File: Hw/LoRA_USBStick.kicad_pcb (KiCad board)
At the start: 2 copper layers, 61.5 x 18.7 mm, 17 parts, among them J10 USB_B, J4 SWD, SW1 RST, U1 ATSAMD21E, U2 RFM95W-868S2, U7 AP2114H-3.3TRG1

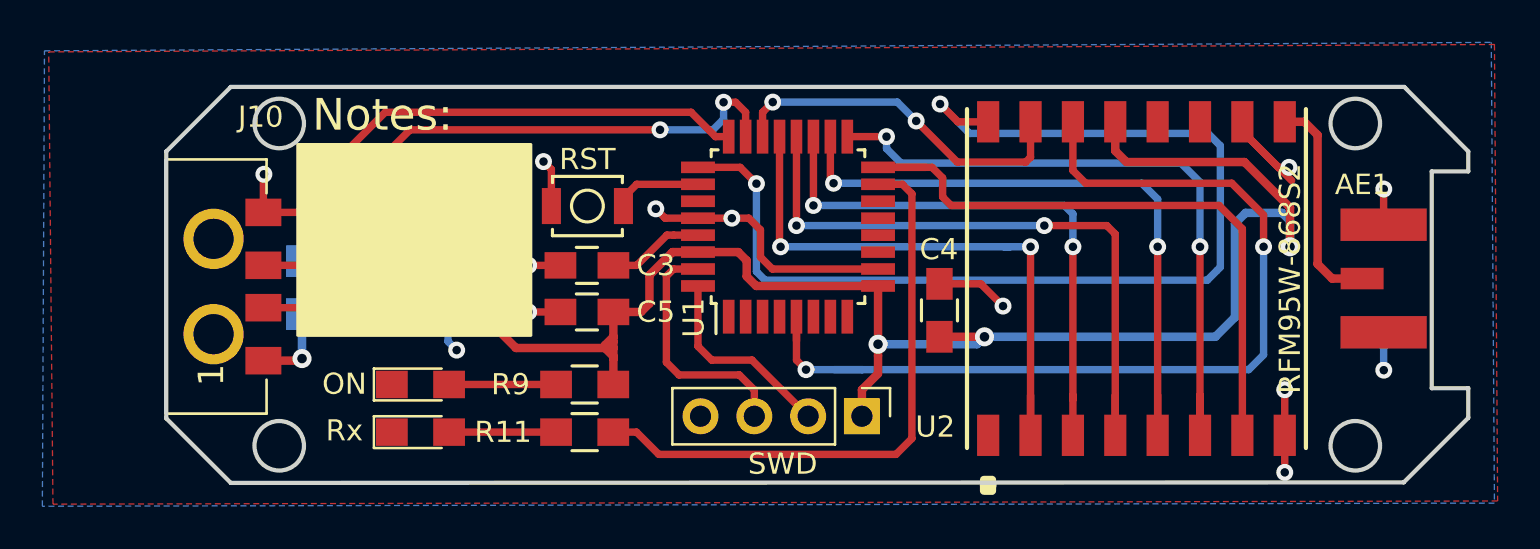
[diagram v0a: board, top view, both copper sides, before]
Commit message: Add v2.0
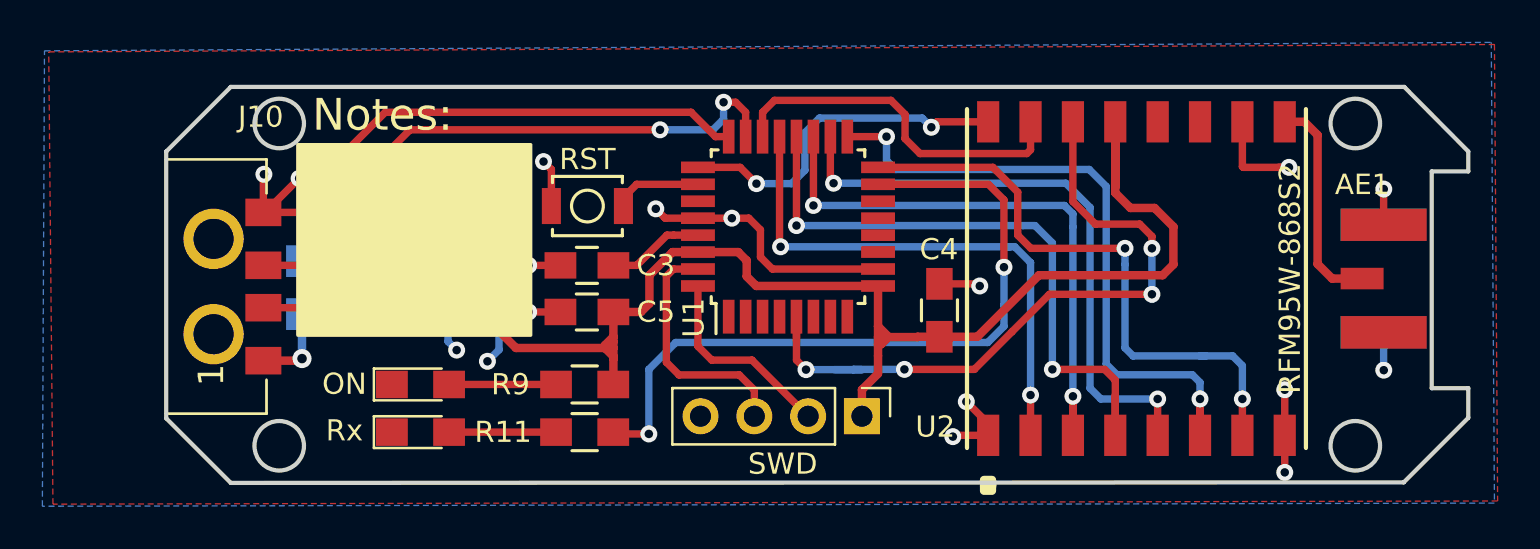
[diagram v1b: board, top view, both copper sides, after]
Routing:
- net /DIO2: track 52.5 -> 17.2 mm
- net /DIO0: track 45.8 -> 34.8 mm, vias 2 -> 4
- net /Rx_LED: track 28.2 -> 34.6 mm, vias 0 -> 2
- net GND: track 41.1 -> 46.7 mm, vias 14 -> 18
- net +3V3: track 92.1 -> 88.8 mm, vias 4 -> 3
- net /DIO5: track 30.9 -> 28.6 mm, vias 0 -> 2
- net /MISO: track 28.1 -> 25.8 mm
- net /SS: track 30.9 -> 28.7 mm
- net /MOSI: track 26.3 -> 28.2 mm
- net /SCK: track 30.8 -> 30.3 mm
- net /DIO1: track 16.9 -> 17.1 mm, vias 2 -> 0
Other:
- net class Default: clearance 0.2 -> 0.3
- rule trace_clearance: 0.2 -> 0.3
